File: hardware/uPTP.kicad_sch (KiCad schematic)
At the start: 1 part, among them U1 CH32V30xWxUx

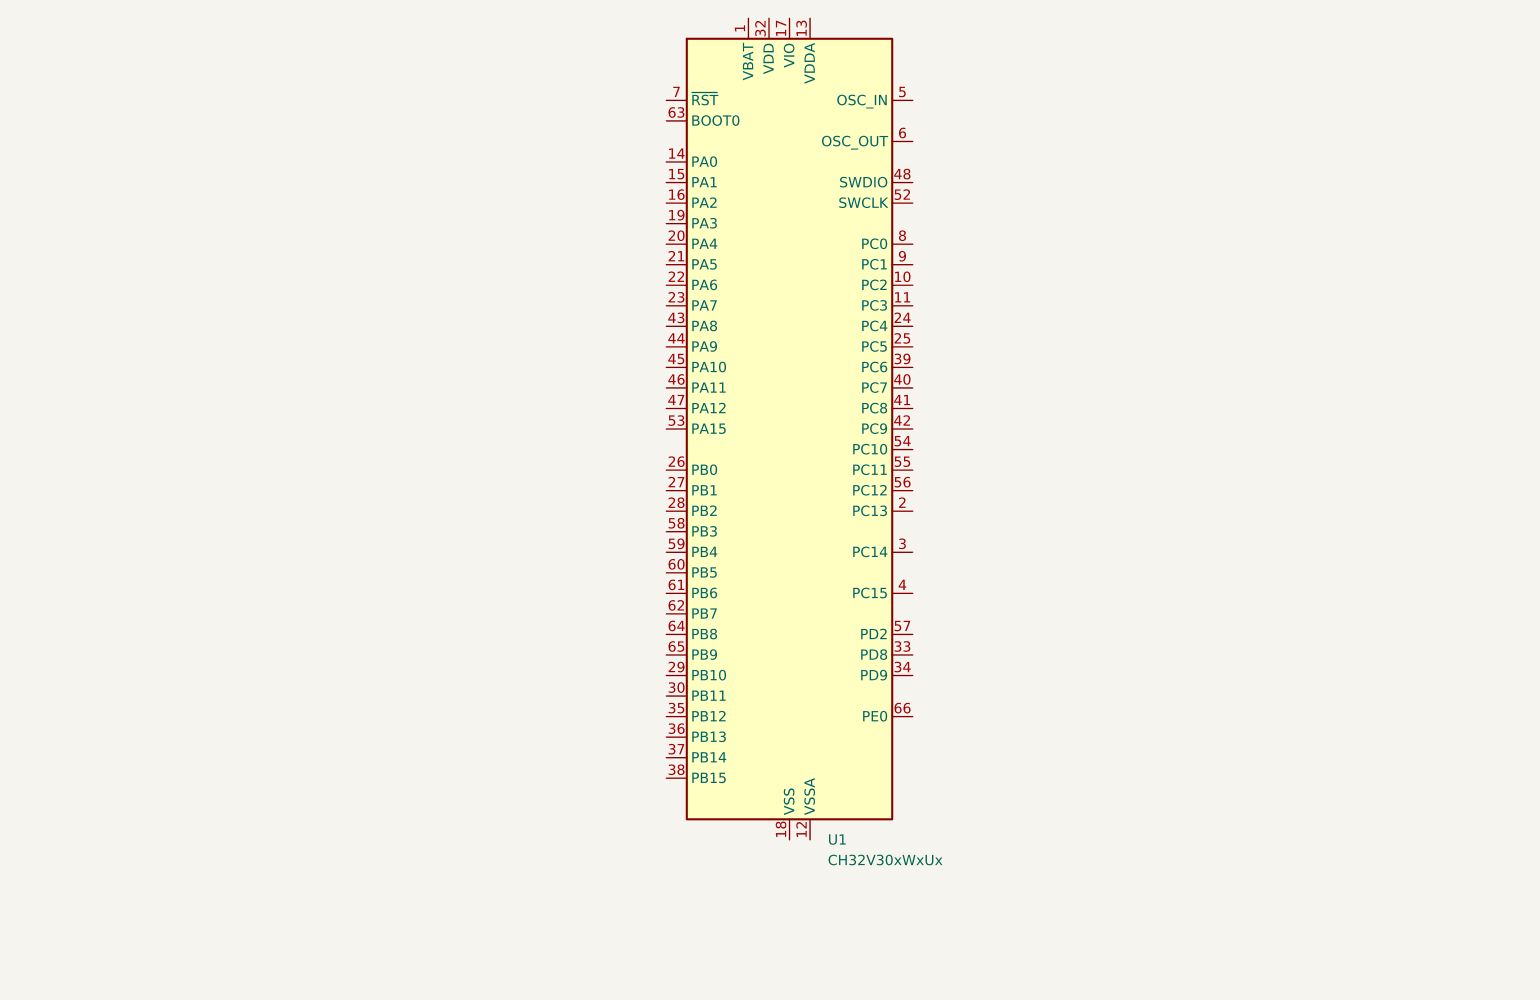
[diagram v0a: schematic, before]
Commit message: Key components
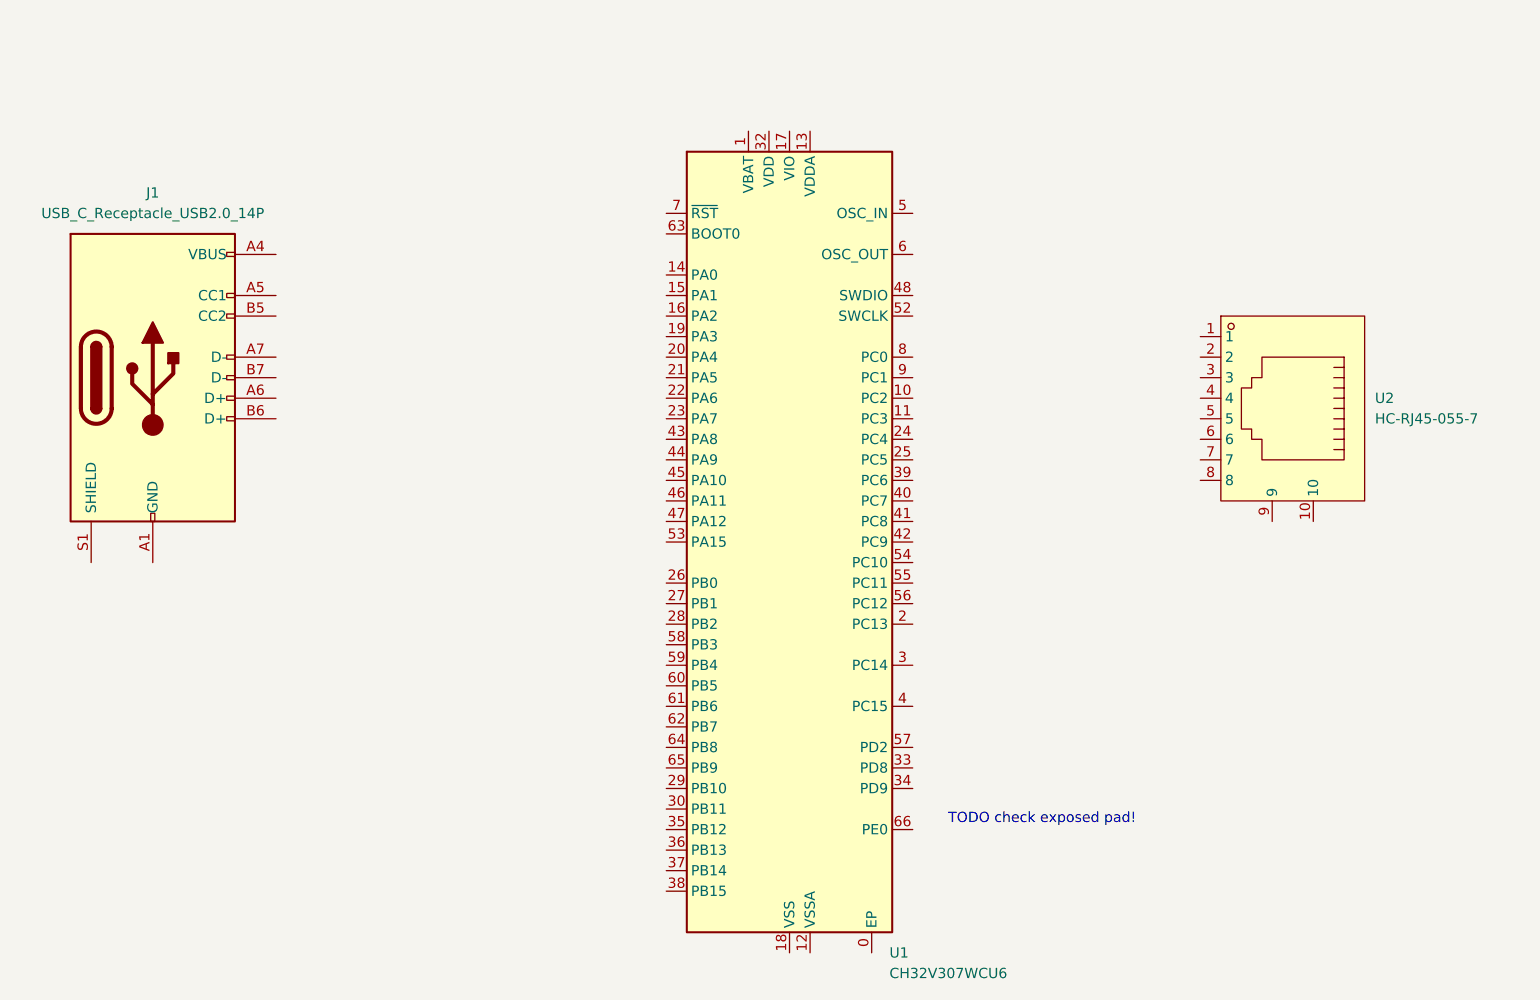
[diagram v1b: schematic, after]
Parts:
- removed U1: CH32V30xWxUx, Package_DFN_QFN:QFN-68-1EP_8x8mm_P0.4mm_EP6.4x6.4mm, symbol MCU_WCH_CH32V3:CH32V30xWxUx
- added J1: USB_C_Receptacle_USB2.0_14P, symbol Connector:USB_C_Receptacle_USB2.0_14P
- added U1: CH32V307WCU6, uPTP:QFN-68_L8.0-W8.0-P0.40-BL-EP6.7, symbol uPTP:CH32V30xWxUx
- added U2: HC-RJ45-055-7, uPTP:RJ45-SMD_HC-RJ45-055-7_1, symbol uPTP:HC-RJ45-055-7
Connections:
- new net: J1.A1 (GND), J1.A12 (GND), J1.B1 (GND), J1.B12 (GND)
- new net: J1.A4 (VBUS), J1.A9 (VBUS), J1.B4 (VBUS), J1.B9 (VBUS)
- new net: U1.17 (VIO), U1.31 (VIO), U1.51 (VIO), U1.67 (VIO)
- new net: U1.18 (VSS), U1.49 (VSS), U1.69 (VSS)
- new net: U1.32 (VDD), U1.50 (VDD), U1.68 (VDD)
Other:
- note added: "TODO check exposed pad!"
